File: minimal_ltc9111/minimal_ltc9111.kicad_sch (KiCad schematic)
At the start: 41 parts, among them J1 FW-02-03-G-D-085-155, J2 FW-02-03-G-D-085-155, J3 FW-02-03-G-D-085-155, Q1 100 V, Q2 100.0 V, Q3 100 V, Q4 100 V, U1 LTC9111RDE-PBF

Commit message: development backup
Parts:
- added C10, C11: 100 pF, capacitor_footprints:C_1812_4532Metric, symbol UNITED_CAPACITORS_DATA_BASE:C_C1812C101JHGACTU
- added D5: 3.3 V, diode_footprints:SOD323, symbol UNITED_DIODES_DATA_BASE:D_SP4020-01FTG-C
- added D6: 58 V, diode_footprints:DO-214AA, symbol UNITED_DIODES_DATA_BASE:D_SMBJ58CA
- added L2: 470 µH, coupled_inductor_footprints:SRF0905A, symbol UNITED_COUPLED_INDUCTORS_DATA_BASE:L_SRF0905A-471Y
- added R7, R8: 10 kΩ, resistor_footprints:R_0603_1608Metric, symbol UNITED_RESISTORS_DATA_BASE:R_ERJ-3EKF1002V
- added R9: 4.7 MΩ, resistor_footprints:R_2010_5025Metric, symbol UNITED_RESISTORS_DATA_BASE:R_CHV2010-JW-475ELF
- added TP7, TP8, TP9: TestPoint, test_point_footprints:TestPoint_THTPad_Castelated, symbol UNITED_TEST_POINTS:TestPoint_Castelated
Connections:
- net GND: now also J2.1, J3.2, R9.2; no longer J2.4, J3.3
- net POWER_IN_N: now also J3.3, L2.4, R8.2; no longer J3.2
- net POWER_IN_P: now also J2.4, L2.2, R7.2; no longer J2.1
- new net: D5.2, D6.1
- new net CABLE+: C10.1, D5.1, L2.3, R7.1, TP7.1
- new net CABLE-: C11.1, D6.2, L2.1, R8.1, TP8.1
- new net Earth: C10.2, C11.2, R9.1, TP9.1
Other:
- moved on the sheet: C1, C2, C3, C4, C5, C6, C7, C8, C9, D1, D2, D3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

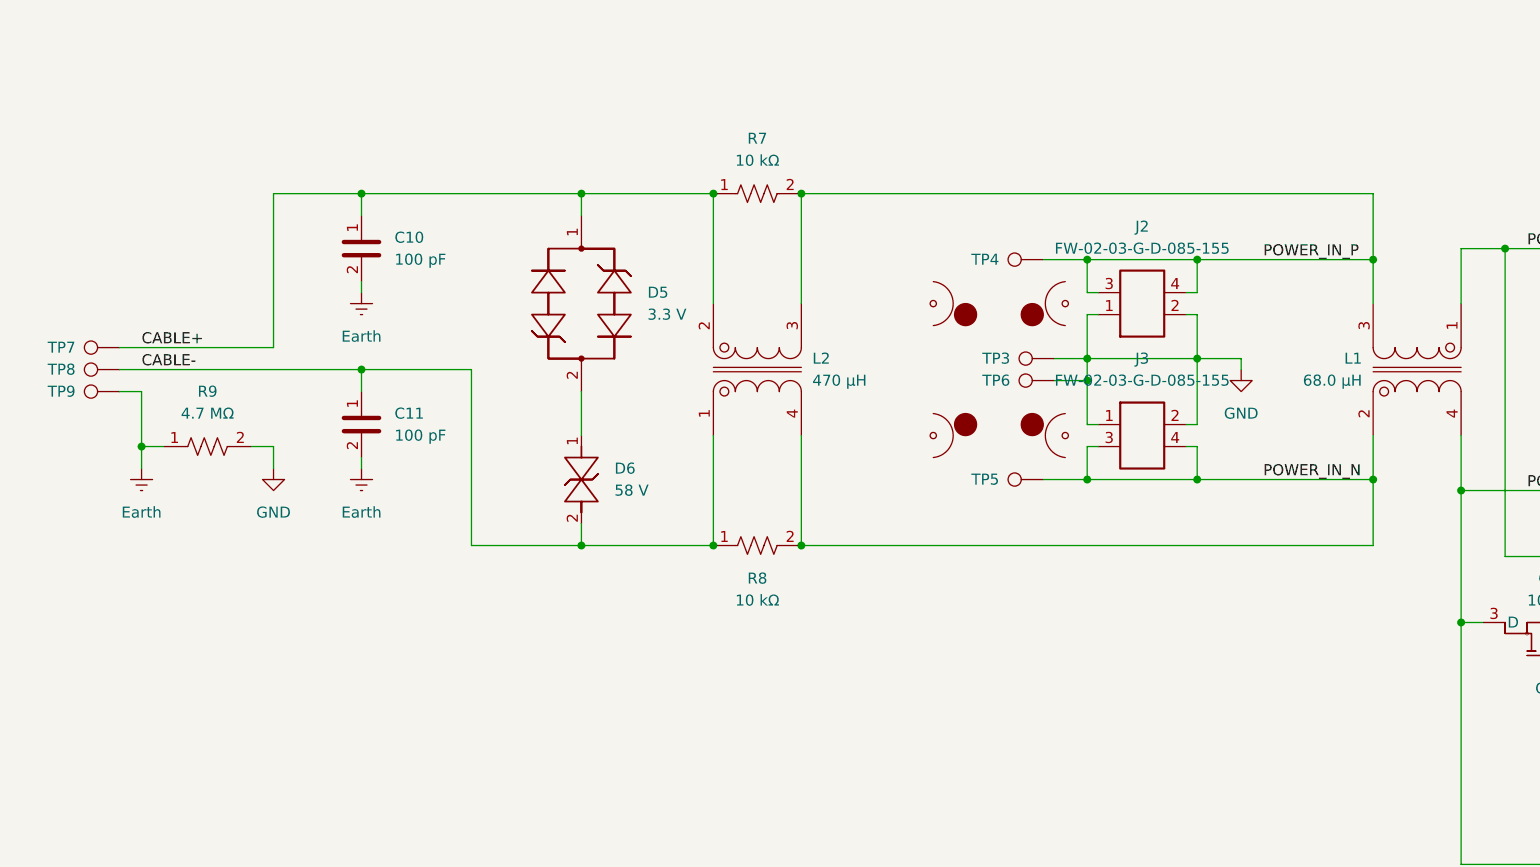
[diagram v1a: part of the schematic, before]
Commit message: development backup
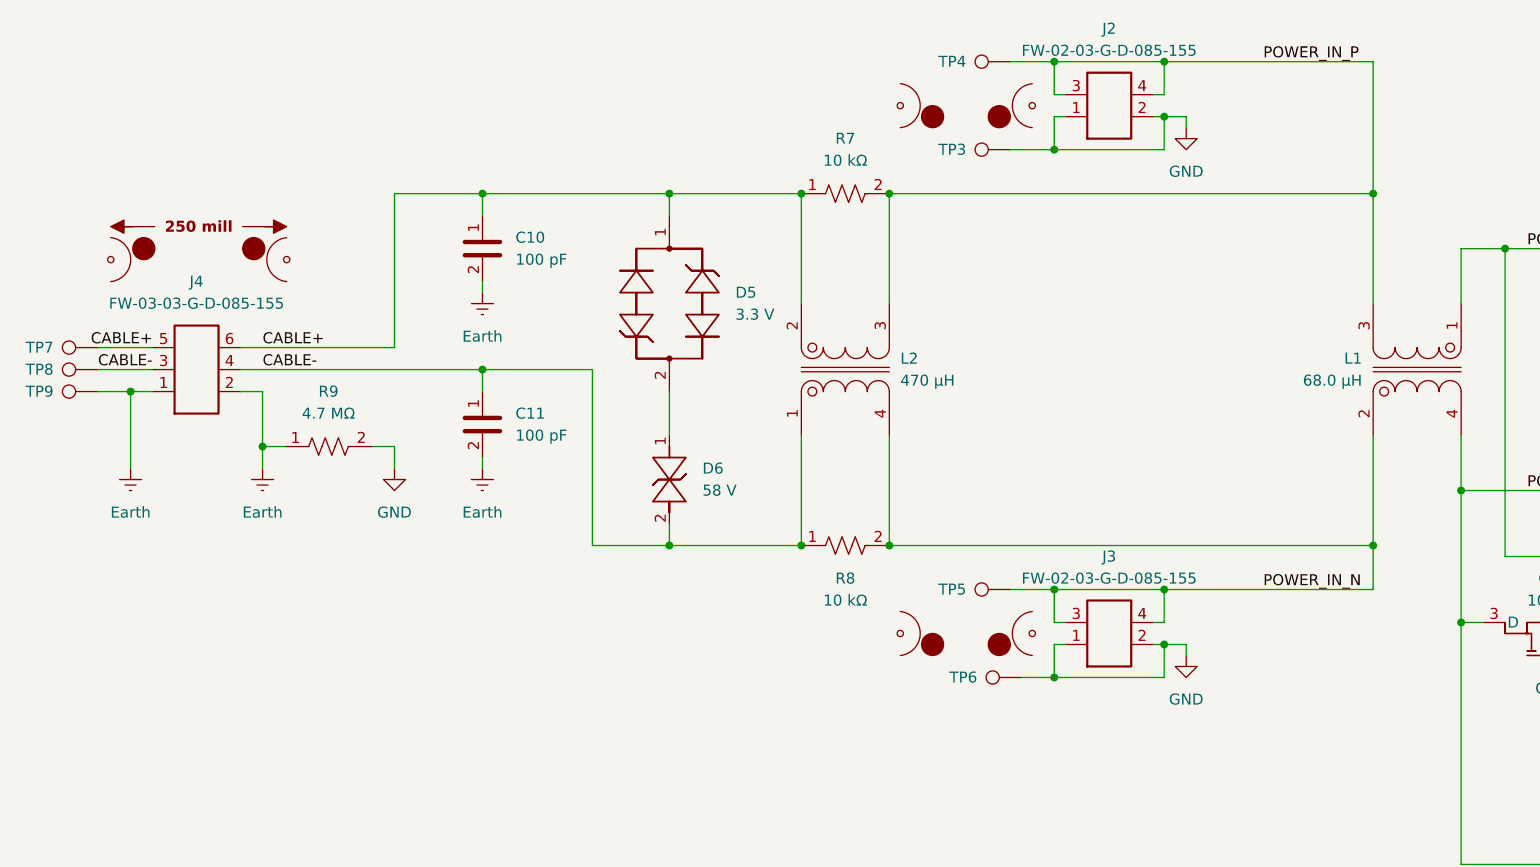
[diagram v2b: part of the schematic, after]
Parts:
- added J4: FW-03-03-G-D-085-155, connector_footprints:FW-03-03-G-D-085-155, symbol UNITED_CONNECTORS_DATA_BASE:J_FW-03-03-G-D-085-155
- added MB6: mouse-bite-50mil-200mil, mouse_bite_footprints:mouse-bite-50mil-250mil, symbol UNITED_MOUSE_BITES_DATA_BASE:mouse-bite-50mil-250mil
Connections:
- net CABLE+: now also J4.5, J4.6
- net CABLE-: now also J4.3, J4.4
- net Earth: now also J4.1, J4.2
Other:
- moved on the sheet: C10, C11, D5, D6, J2, J3, L2, R7, R8, R9, TP3, TP4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
